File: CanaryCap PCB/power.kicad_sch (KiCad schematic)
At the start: 8 parts, among them U2 LM3940 3.3V-SOT223, U4 LMZM23601V5

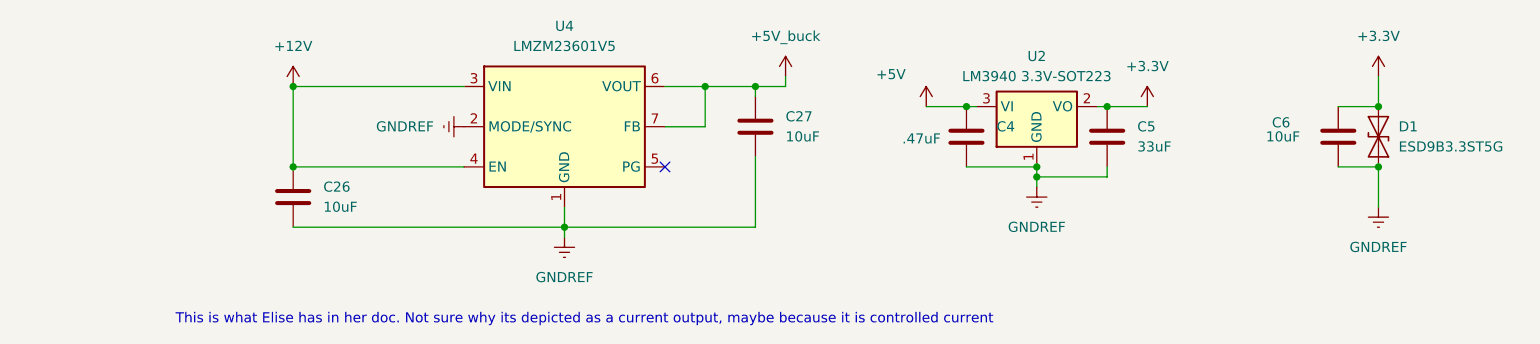
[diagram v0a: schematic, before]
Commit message: FIXED IT MF
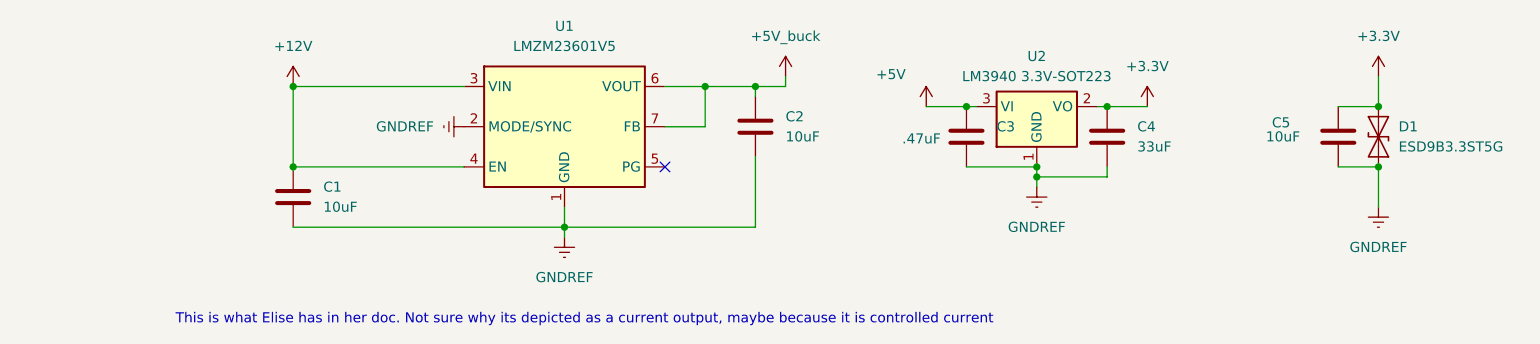
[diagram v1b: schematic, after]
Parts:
- renumbered C26 to C1, C27 to C2, C4 to C3, C5 to C4, C6 to C5, U4 to U1
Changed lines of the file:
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@@
 		(dnp no)
 		(fields_autoplaced yes)
-		(property "Reference" "#PWR08"
+		(property "Reference" "#PWR07"
 			(at 160.02 85.09 0)
 			(effects
@@
 			(project "CanaryCap"
 				(path "/406ad30e-b04c-4bb7-9588-aab8ab73084a/3219e357-ed27-4a99-8f08-f1a850fa8309"
-					(reference "#PWR08")
+					(reference "#PWR07")
 					(unit 1)
 				)
@@
 		(dnp no)
 		(fields_autoplaced yes)
-		(property "Reference" "C26"
+		(property "Reference" "C1"
 			(at 55.88 91.4399 0)
 			(effects
@@
 			(project "CanaryCap"
 				(path "/406ad30e-b04c-4bb7-9588-aab8ab73084a/3219e357-ed27-4a99-8f08-f1a850fa8309"
-					(reference "C26")
+					(reference "C1")
 					(unit 1)
 				)
@@
 		(dnp no)
 		(fields_autoplaced yes)
-		(property "Reference" "#PWR039"
+		(property "Reference" "#PWR02"
 			(at 67.31 83.82 0)
 			(effects
@@
 			(project "CanaryCap"
 				(path "/406ad30e-b04c-4bb7-9588-aab8ab73084a/3219e357-ed27-4a99-8f08-f1a850fa8309"
-					(reference "#PWR039")
+					(reference "#PWR02")
 					(unit 1)
 				)
@@
 		(dnp no)
 		(fields_autoplaced yes)
-		(property "Reference" "#PWR09"
+		(property "Reference" "#PWR08"
 			(at 189.23 81.28 0)
 			(effects
@@
 			(project "CanaryCap"
 				(path "/406ad30e-b04c-4bb7-9588-aab8ab73084a/3219e357-ed27-4a99-8f08-f1a850fa8309"
-					(reference "#PWR09")
+					(reference "#PWR08")
 					(unit 1)
 				)
@@
 		(dnp no)
 		(fields_autoplaced yes)
-		(property "Reference" "U4"
+		(property "Reference" "U1"
 			(at 86.36 71.12 0)
 			(effects
@@
 			(project ""
 				(path "/406ad30e-b04c-4bb7-9588-aab8ab73084a/3219e357-ed27-4a99-8f08-f1a850fa8309"
-					(reference "U4")
+					(reference "U1")
 					(unit 1)
 				)
@@
 		(on_board yes)
 		(dnp no)
-		(property "Reference" "#PWR06"
+		(property "Reference" "#PWR05"
 			(at 132.08 85.09 0)
 			(effects
@@
 			(project "CanaryCap"
 				(path "/406ad30e-b04c-4bb7-9588-aab8ab73084a/3219e357-ed27-4a99-8f08-f1a850fa8309"
-					(reference "#PWR06")
+					(reference "#PWR05")
 					(unit 1)
 				)
@@
 		(on_board yes)
 		(dnp no)
-		(property "Reference" "C6"
+		(property "Reference" "C5"
 			(at 175.768 83.312 0)
 			(effects
@@
 			(project "CanaryCap"
 				(path "/406ad30e-b04c-4bb7-9588-aab8ab73084a/3219e357-ed27-4a99-8f08-f1a850fa8309"
-					(reference "C6")
+					(reference "C5")
 					(unit 1)
 				)
@@
 		(dnp no)
 		(fields_autoplaced yes)
-		(property "Reference" "#PWR010"
+		(property "Reference" "#PWR09"
 			(at 189.23 100.33 0)
 			(effects
@@
 			(project "CanaryCap"
 				(path "/406ad30e-b04c-4bb7-9588-aab8ab73084a/3219e357-ed27-4a99-8f08-f1a850fa8309"
-					(reference "#PWR010")
+					(reference "#PWR09")
 					(unit 1)
 				)
@@
 		(on_board yes)
 		(dnp no)
-		(property "Reference" "C4"
+		(property "Reference" "C3"
 			(at 140.97 83.8199 0)
 			(effects
@@
 			(project "CanaryCap"
 				(path "/406ad30e-b04c-4bb7-9588-aab8ab73084a/3219e357-ed27-4a99-8f08-f1a850fa8309"
-					(reference "C4")
+					(reference "C3")
 					(unit 1)
 				)
@@
 		(dnp no)
 		(fields_autoplaced yes)
-		(property "Reference" "#PWR036"
+		(property "Reference" "#PWR01"
 			(at 52.07 82.55 0)
 			(effects
@@
 			(project "CanaryCap"
 				(path "/406ad30e-b04c-4bb7-9588-aab8ab73084a/3219e357-ed27-4a99-8f08-f1a850fa8309"
-					(reference "#PWR036")
+					(reference "#PWR01")
 					(unit 1)
 				)
@@
 		(dnp no)
 		(fields_autoplaced yes)
-		(property "Reference" "#PWR035"
+		(property "Reference" "#PWR03"
 			(at 86.36 104.14 0)
 			(effects
@@
 			(project "CanaryCap"
 				(path "/406ad30e-b04c-4bb7-9588-aab8ab73084a/3219e357-ed27-4a99-8f08-f1a850fa8309"
-					(reference "#PWR035")
+					(reference "#PWR03")
 					(unit 1)
 				)
@@
 		(dnp no)
 		(fields_autoplaced yes)
-		(property "Reference" "#PWR07"
+		(property "Reference" "#PWR06"
 			(at 146.05 97.79 0)
 			(effects
@@
 			(project "CanaryCap"
 				(path "/406ad30e-b04c-4bb7-9588-aab8ab73084a/3219e357-ed27-4a99-8f08-f1a850fa8309"
-					(reference "#PWR07")
+					(reference "#PWR06")
 					(unit 1)
 				)
@@
 		(dnp no)
 		(fields_autoplaced yes)
-		(property "Reference" "C5"
+		(property "Reference" "C4"
 			(at 158.75 83.8199 0)
 			(effects
@@
 			(project "CanaryCap"
 				(path "/406ad30e-b04c-4bb7-9588-aab8ab73084a/3219e357-ed27-4a99-8f08-f1a850fa8309"
-					(reference "C5")
+					(reference "C4")
 					(unit 1)
 				)
@@
 		(dnp no)
 		(fields_autoplaced yes)
-		(property "Reference" "#PWR037"
+		(property "Reference" "#PWR04"
 			(at 114.3 81.28 0)
 			(effects
@@
 			(project "CanaryCap"
 				(path "/406ad30e-b04c-4bb7-9588-aab8ab73084a/3219e357-ed27-4a99-8f08-f1a850fa8309"
-					(reference "#PWR037")
+					(reference "#PWR04")
 					(unit 1)
 				)
@@
 		(dnp no)
 		(fields_autoplaced yes)
-		(property "Reference" "C27"
+		(property "Reference" "C2"
 			(at 114.3 82.5499 0)
 			(effects
@@
 			(project "CanaryCap"
 				(path "/406ad30e-b04c-4bb7-9588-aab8ab73084a/3219e357-ed27-4a99-8f08-f1a850fa8309"
-					(reference "C27")
-					(unit 1)
-				)
+					(reference "C2")
+					(unit 1)
+				)

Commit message: Added todo
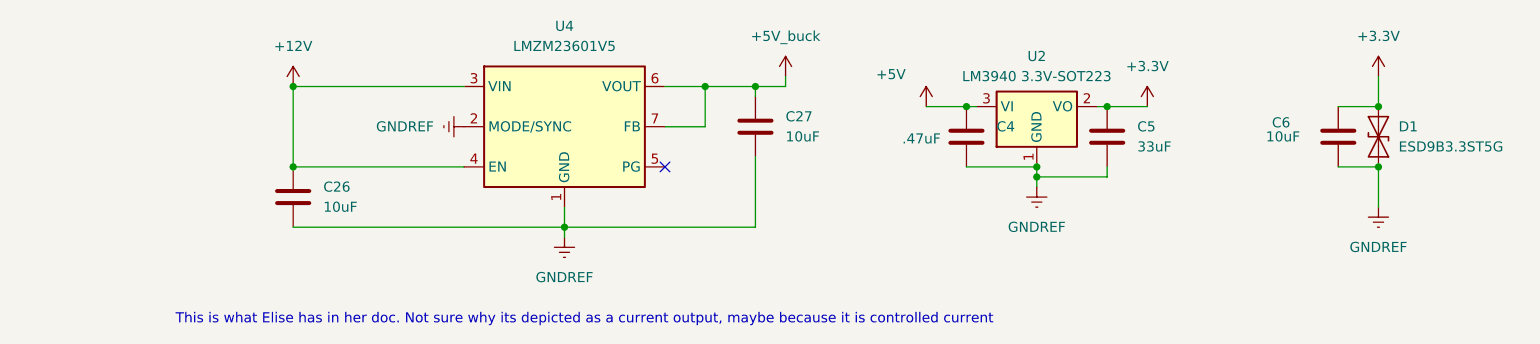
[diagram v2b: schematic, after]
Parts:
- renumbered C1 to C26, C2 to C27, C3 to C4, C4 to C5, C5 to C6, U1 to U4
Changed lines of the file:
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@@
 		(dnp no)
 		(fields_autoplaced yes)
-		(property "Reference" "#PWR07"
+		(property "Reference" "#PWR08"
 			(at 160.02 85.09 0)
 			(effects
@@
 			(project "CanaryCap"
 				(path "/406ad30e-b04c-4bb7-9588-aab8ab73084a/3219e357-ed27-4a99-8f08-f1a850fa8309"
-					(reference "#PWR07")
+					(reference "#PWR08")
 					(unit 1)
 				)
@@
 		(dnp no)
 		(fields_autoplaced yes)
-		(property "Reference" "C1"
+		(property "Reference" "C26"
 			(at 55.88 91.4399 0)
 			(effects
@@
 			(project "CanaryCap"
 				(path "/406ad30e-b04c-4bb7-9588-aab8ab73084a/3219e357-ed27-4a99-8f08-f1a850fa8309"
-					(reference "C1")
+					(reference "C26")
 					(unit 1)
 				)
@@
 		(dnp no)
 		(fields_autoplaced yes)
-		(property "Reference" "#PWR02"
+		(property "Reference" "#PWR039"
 			(at 67.31 83.82 0)
 			(effects
@@
 			(project "CanaryCap"
 				(path "/406ad30e-b04c-4bb7-9588-aab8ab73084a/3219e357-ed27-4a99-8f08-f1a850fa8309"
-					(reference "#PWR02")
+					(reference "#PWR039")
 					(unit 1)
 				)
@@
 		(dnp no)
 		(fields_autoplaced yes)
-		(property "Reference" "#PWR08"
+		(property "Reference" "#PWR09"
 			(at 189.23 81.28 0)
 			(effects
@@
 			(project "CanaryCap"
 				(path "/406ad30e-b04c-4bb7-9588-aab8ab73084a/3219e357-ed27-4a99-8f08-f1a850fa8309"
-					(reference "#PWR08")
+					(reference "#PWR09")
 					(unit 1)
 				)
@@
 		(dnp no)
 		(fields_autoplaced yes)
-		(property "Reference" "U1"
+		(property "Reference" "U4"
 			(at 86.36 71.12 0)
 			(effects
@@
 			(project ""
 				(path "/406ad30e-b04c-4bb7-9588-aab8ab73084a/3219e357-ed27-4a99-8f08-f1a850fa8309"
-					(reference "U1")
+					(reference "U4")
 					(unit 1)
 				)
@@
 		(on_board yes)
 		(dnp no)
-		(property "Reference" "#PWR05"
+		(property "Reference" "#PWR06"
 			(at 132.08 85.09 0)
 			(effects
@@
 			(project "CanaryCap"
 				(path "/406ad30e-b04c-4bb7-9588-aab8ab73084a/3219e357-ed27-4a99-8f08-f1a850fa8309"
-					(reference "#PWR05")
+					(reference "#PWR06")
 					(unit 1)
 				)
@@
 		(on_board yes)
 		(dnp no)
-		(property "Reference" "C5"
+		(property "Reference" "C6"
 			(at 175.768 83.312 0)
 			(effects
@@
 			(project "CanaryCap"
 				(path "/406ad30e-b04c-4bb7-9588-aab8ab73084a/3219e357-ed27-4a99-8f08-f1a850fa8309"
-					(reference "C5")
+					(reference "C6")
 					(unit 1)
 				)
@@
 		(dnp no)
 		(fields_autoplaced yes)
-		(property "Reference" "#PWR09"
+		(property "Reference" "#PWR010"
 			(at 189.23 100.33 0)
 			(effects
@@
 			(project "CanaryCap"
 				(path "/406ad30e-b04c-4bb7-9588-aab8ab73084a/3219e357-ed27-4a99-8f08-f1a850fa8309"
-					(reference "#PWR09")
+					(reference "#PWR010")
 					(unit 1)
 				)
@@
 		(on_board yes)
 		(dnp no)
-		(property "Reference" "C3"
+		(property "Reference" "C4"
 			(at 140.97 83.8199 0)
 			(effects
@@
 			(project "CanaryCap"
 				(path "/406ad30e-b04c-4bb7-9588-aab8ab73084a/3219e357-ed27-4a99-8f08-f1a850fa8309"
-					(reference "C3")
+					(reference "C4")
 					(unit 1)
 				)
@@
 		(dnp no)
 		(fields_autoplaced yes)
-		(property "Reference" "#PWR01"
+		(property "Reference" "#PWR036"
 			(at 52.07 82.55 0)
 			(effects
@@
 			(project "CanaryCap"
 				(path "/406ad30e-b04c-4bb7-9588-aab8ab73084a/3219e357-ed27-4a99-8f08-f1a850fa8309"
-					(reference "#PWR01")
+					(reference "#PWR036")
 					(unit 1)
 				)
@@
 		(dnp no)
 		(fields_autoplaced yes)
-		(property "Reference" "#PWR03"
+		(property "Reference" "#PWR035"
 			(at 86.36 104.14 0)
 			(effects
@@
 			(project "CanaryCap"
 				(path "/406ad30e-b04c-4bb7-9588-aab8ab73084a/3219e357-ed27-4a99-8f08-f1a850fa8309"
-					(reference "#PWR03")
+					(reference "#PWR035")
 					(unit 1)
 				)
@@
 		(dnp no)
 		(fields_autoplaced yes)
-		(property "Reference" "#PWR06"
+		(property "Reference" "#PWR07"
 			(at 146.05 97.79 0)
 			(effects
@@
 			(project "CanaryCap"
 				(path "/406ad30e-b04c-4bb7-9588-aab8ab73084a/3219e357-ed27-4a99-8f08-f1a850fa8309"
-					(reference "#PWR06")
+					(reference "#PWR07")
 					(unit 1)
 				)
@@
 		(dnp no)
 		(fields_autoplaced yes)
-		(property "Reference" "C4"
+		(property "Reference" "C5"
 			(at 158.75 83.8199 0)
 			(effects
@@
 			(project "CanaryCap"
 				(path "/406ad30e-b04c-4bb7-9588-aab8ab73084a/3219e357-ed27-4a99-8f08-f1a850fa8309"
-					(reference "C4")
+					(reference "C5")
 					(unit 1)
 				)
@@
 		(dnp no)
 		(fields_autoplaced yes)
-		(property "Reference" "#PWR04"
+		(property "Reference" "#PWR037"
 			(at 114.3 81.28 0)
 			(effects
@@
 			(project "CanaryCap"
 				(path "/406ad30e-b04c-4bb7-9588-aab8ab73084a/3219e357-ed27-4a99-8f08-f1a850fa8309"
-					(reference "#PWR04")
+					(reference "#PWR037")
 					(unit 1)
 				)
@@
 		(dnp no)
 		(fields_autoplaced yes)
-		(property "Reference" "C2"
+		(property "Reference" "C27"
 			(at 114.3 82.5499 0)
 			(effects
@@
 			(project "CanaryCap"
 				(path "/406ad30e-b04c-4bb7-9588-aab8ab73084a/3219e357-ed27-4a99-8f08-f1a850fa8309"
-					(reference "C2")
-					(unit 1)
-				)
+					(reference "C27")
+					(unit 1)
+				)
